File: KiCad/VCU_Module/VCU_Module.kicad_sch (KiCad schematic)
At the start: 45 parts, among them J1 5810132011, J10 12V, J12 MCU1, J13 MCU2, J14 5V, J15 3V3, J16 MCU3, J17 MCU4, J2 CN1, J3 CN2, J4 CN3, J5 MCU6, J6 CN4, J7 MCU5, J9 GND, Q1 SUD19P06-60, U3 LMR33640DDDA, U4 LMR33640DDDA

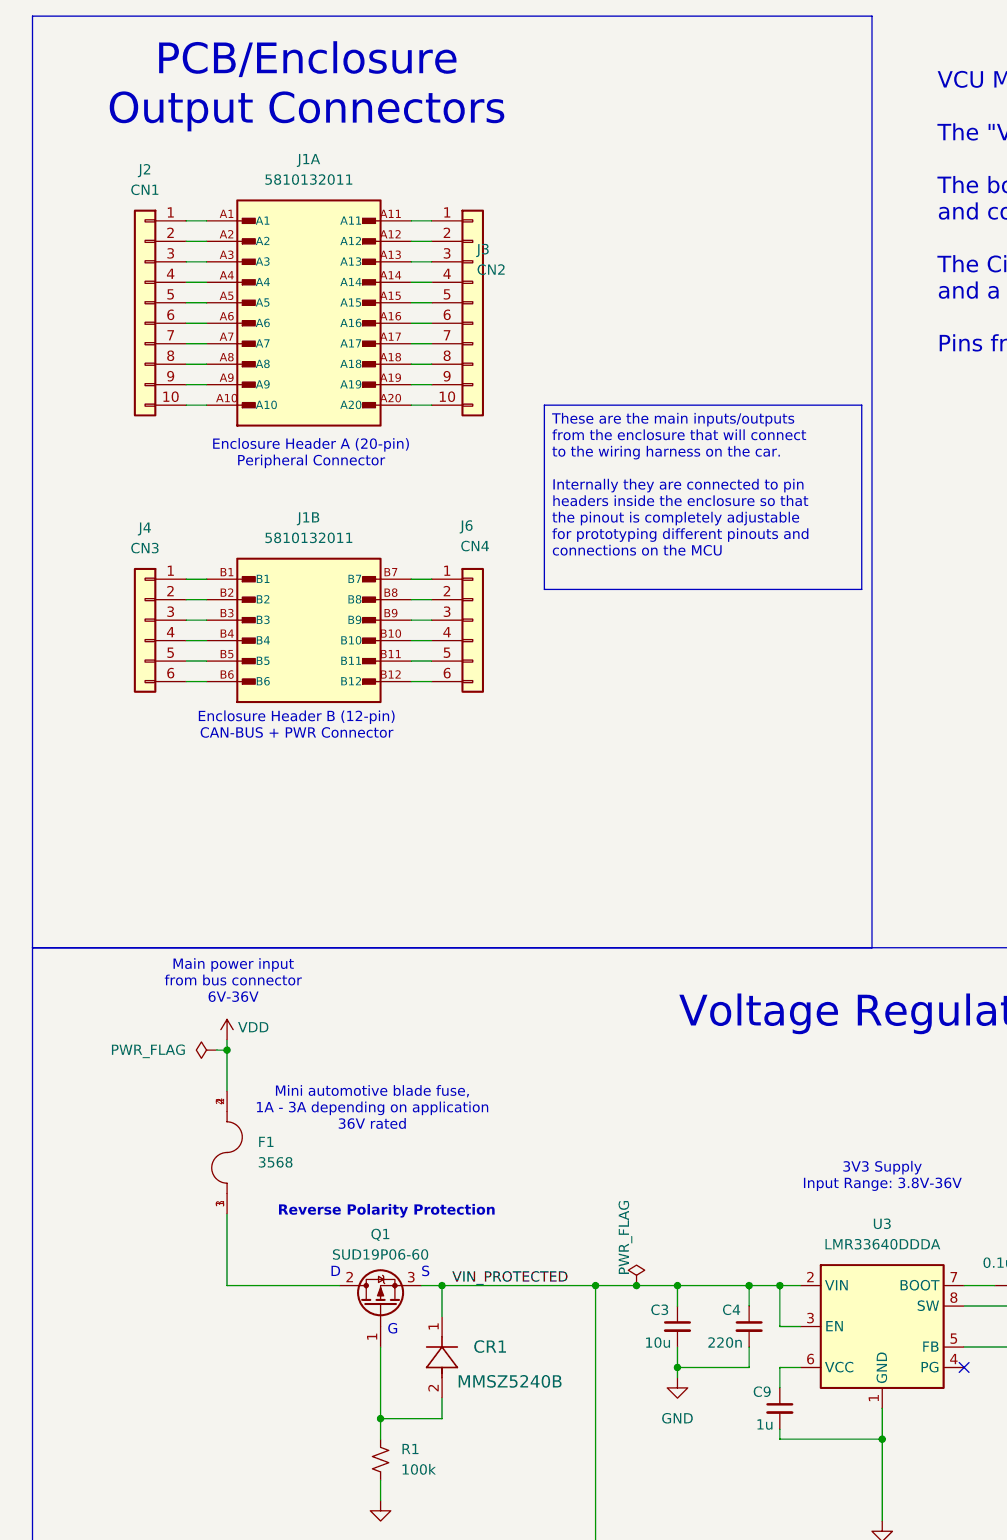
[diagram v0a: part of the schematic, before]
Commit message: final PCB fix
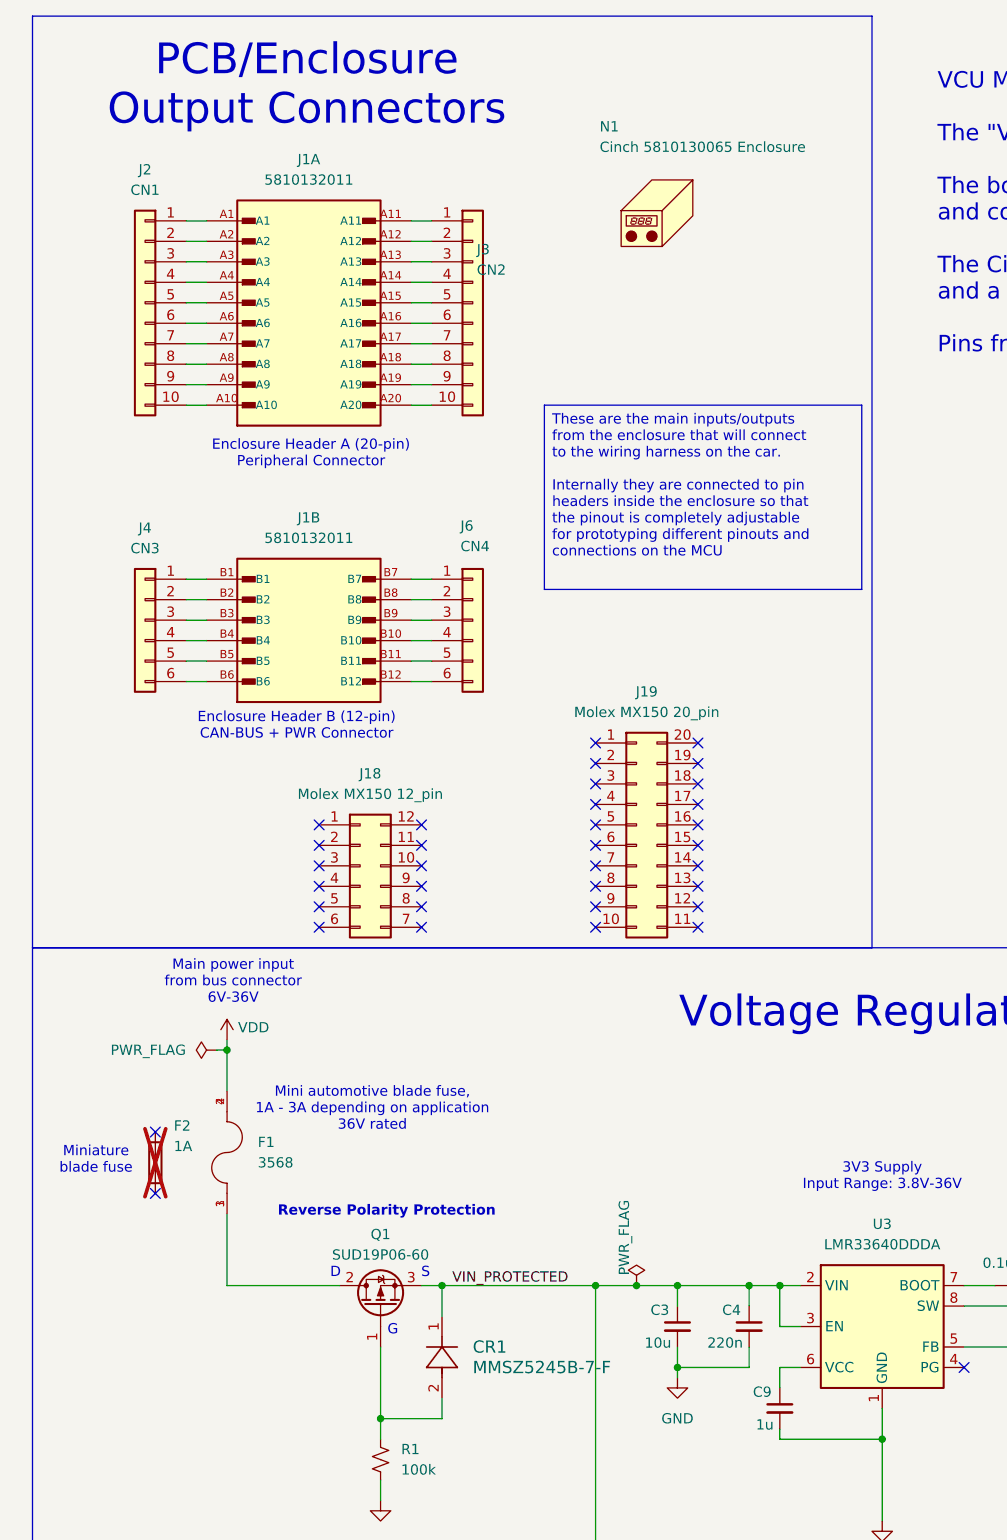
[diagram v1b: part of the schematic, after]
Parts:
- removed CR1: MMSZ5240B, VMS_Footprints:SOD123_DIO, symbol MMSZ5245B_7_F:MMSZ5245B-7-F
- added CR1: MMSZ5245B-7-F, VMS_Footprints:SOD123_DIO, symbol VMS_Symbols:MMSZ5245B-7-F
- added F2: 1A, symbol Device:Fuse
- added J18: Molex MX150 12_pin, N/A, symbol Connector_Generic:Conn_02x06_Counter_Clockwise
- added J19: Molex MX150 20_pin, N/A, symbol Connector_Generic:Conn_02x10_Counter_Clockwise
- added N1: Cinch 5810130065 Enclosure, N/A, symbol Mechanical:Housing
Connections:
- net VIN_PROTECTED: now also CR1.1
- net at Q1.1 (G), R1.1: now also CR1.2
- no-connect marks 2 -> 36
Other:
- note added: "Miniature blade fuse"
